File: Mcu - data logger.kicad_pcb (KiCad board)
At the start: 2 copper layers, 52.8 x 34.3 mm, 29 parts, among them J1 Conn_01x04_Pin, J2 Conn_01x09_Pin, J3 Conn_01x04_Pin, J4 Conn_02x03_Odd_Even, U1 24LC1025, U2 DS1337S_, U3 24LC1025, U4 ATMEGA328P-AU, Y1 32.768 KHz, Y2 16 MHz

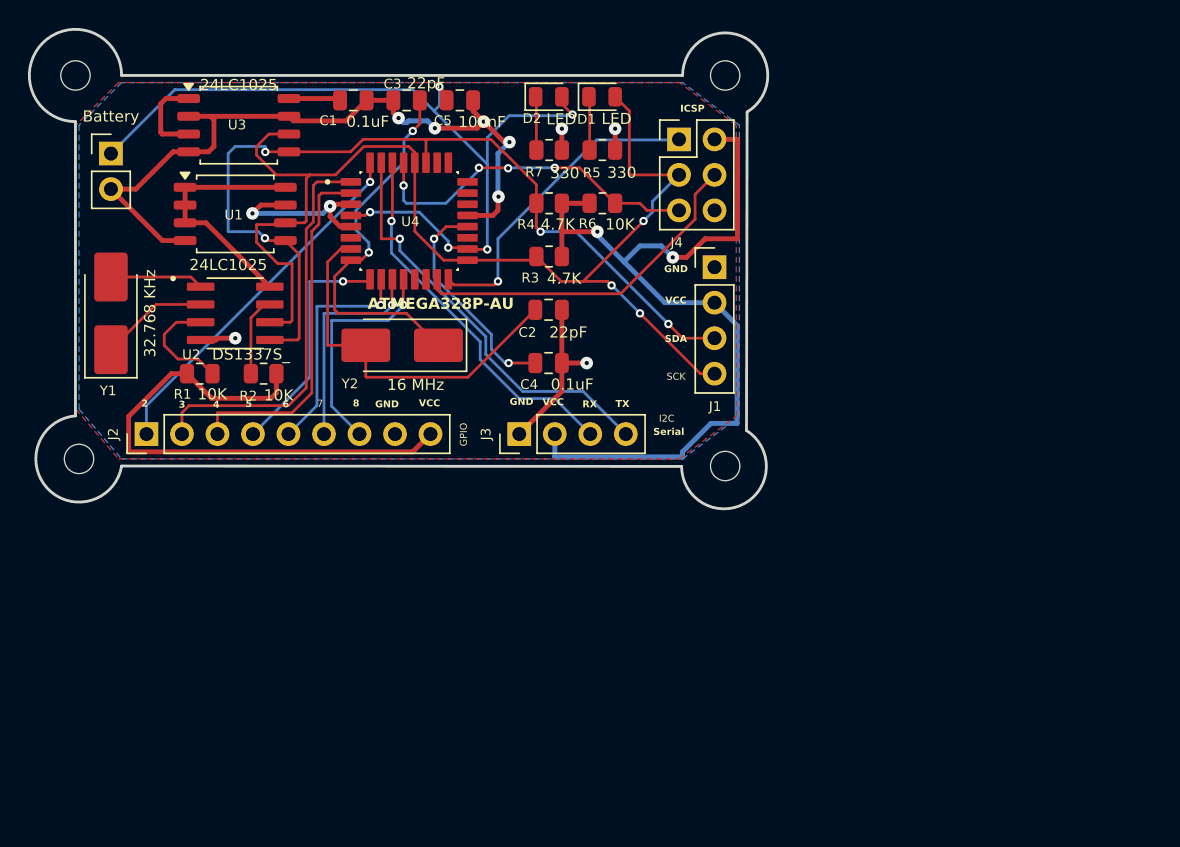
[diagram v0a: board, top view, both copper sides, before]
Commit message: Layout design done
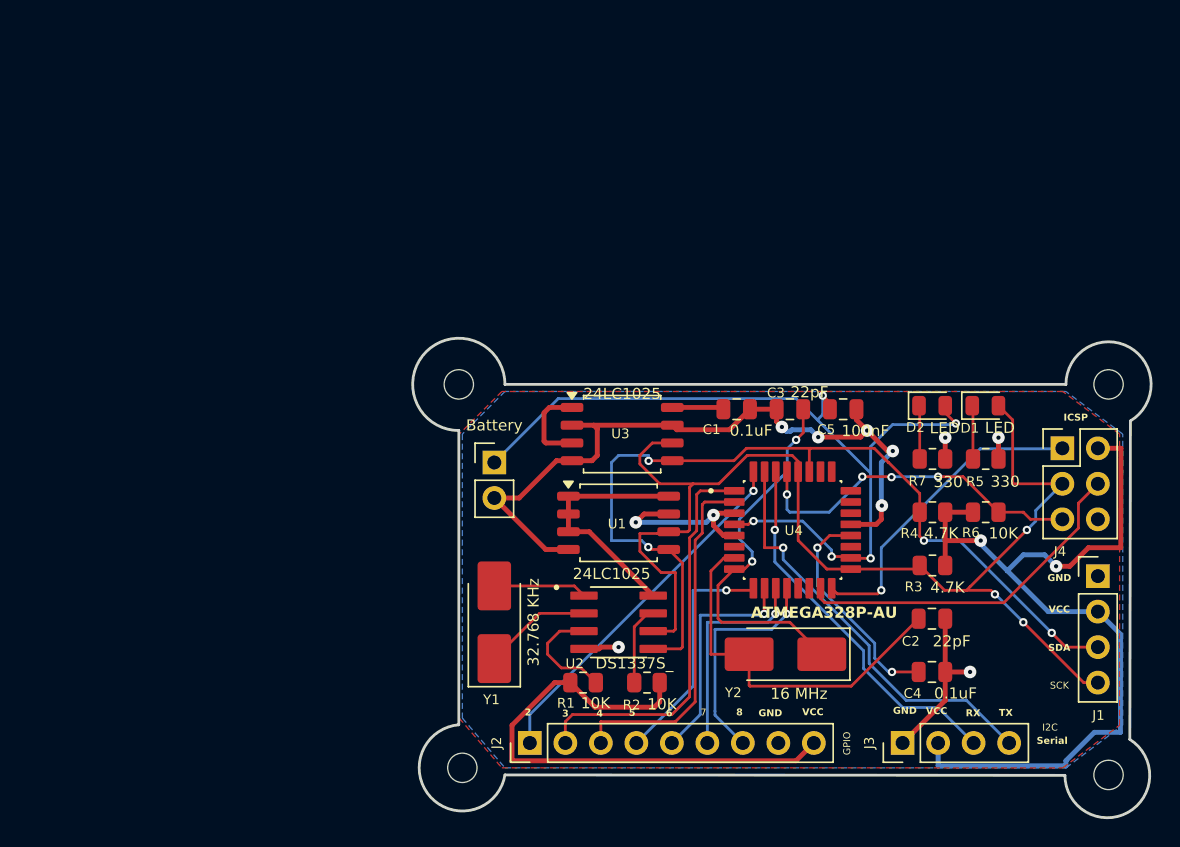
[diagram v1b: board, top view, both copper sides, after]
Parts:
- moved J2 35.2 mm to (66.8, 104.7)
- moved U3 35.2 mm to (73.4, 82.6)
- moved BT1 35.2 mm to (64.3, 84.6)
- moved C1 35.2 mm to (81.6, 80.8)
- moved C2 35.2 mm to (95.6, 95.8)
- moved C3 35.2 mm to (85.4, 80.8)
- moved C5 35.2 mm to (89.2, 80.8)
- moved D2 35.2 mm to (95.6, 80.5)
- moved H4 35.2 mm to (108.2, 106.9)
- moved J1 35.2 mm to (107.4, 92.7)
- moved J3 35.2 mm to (93.5, 104.7)
- moved R3 35.2 mm to (95.6, 92.0)
- moved R5 35.2 mm to (99.4, 84.3)
- moved R7 35.2 mm to (95.6, 84.3)
- moved C4 35.2 mm to (95.6, 99.6)
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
